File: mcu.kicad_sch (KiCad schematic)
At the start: 9 parts, among them SW1 SW_MEC_5E, U9 ESP32-S3-WROOM-1-N16R8

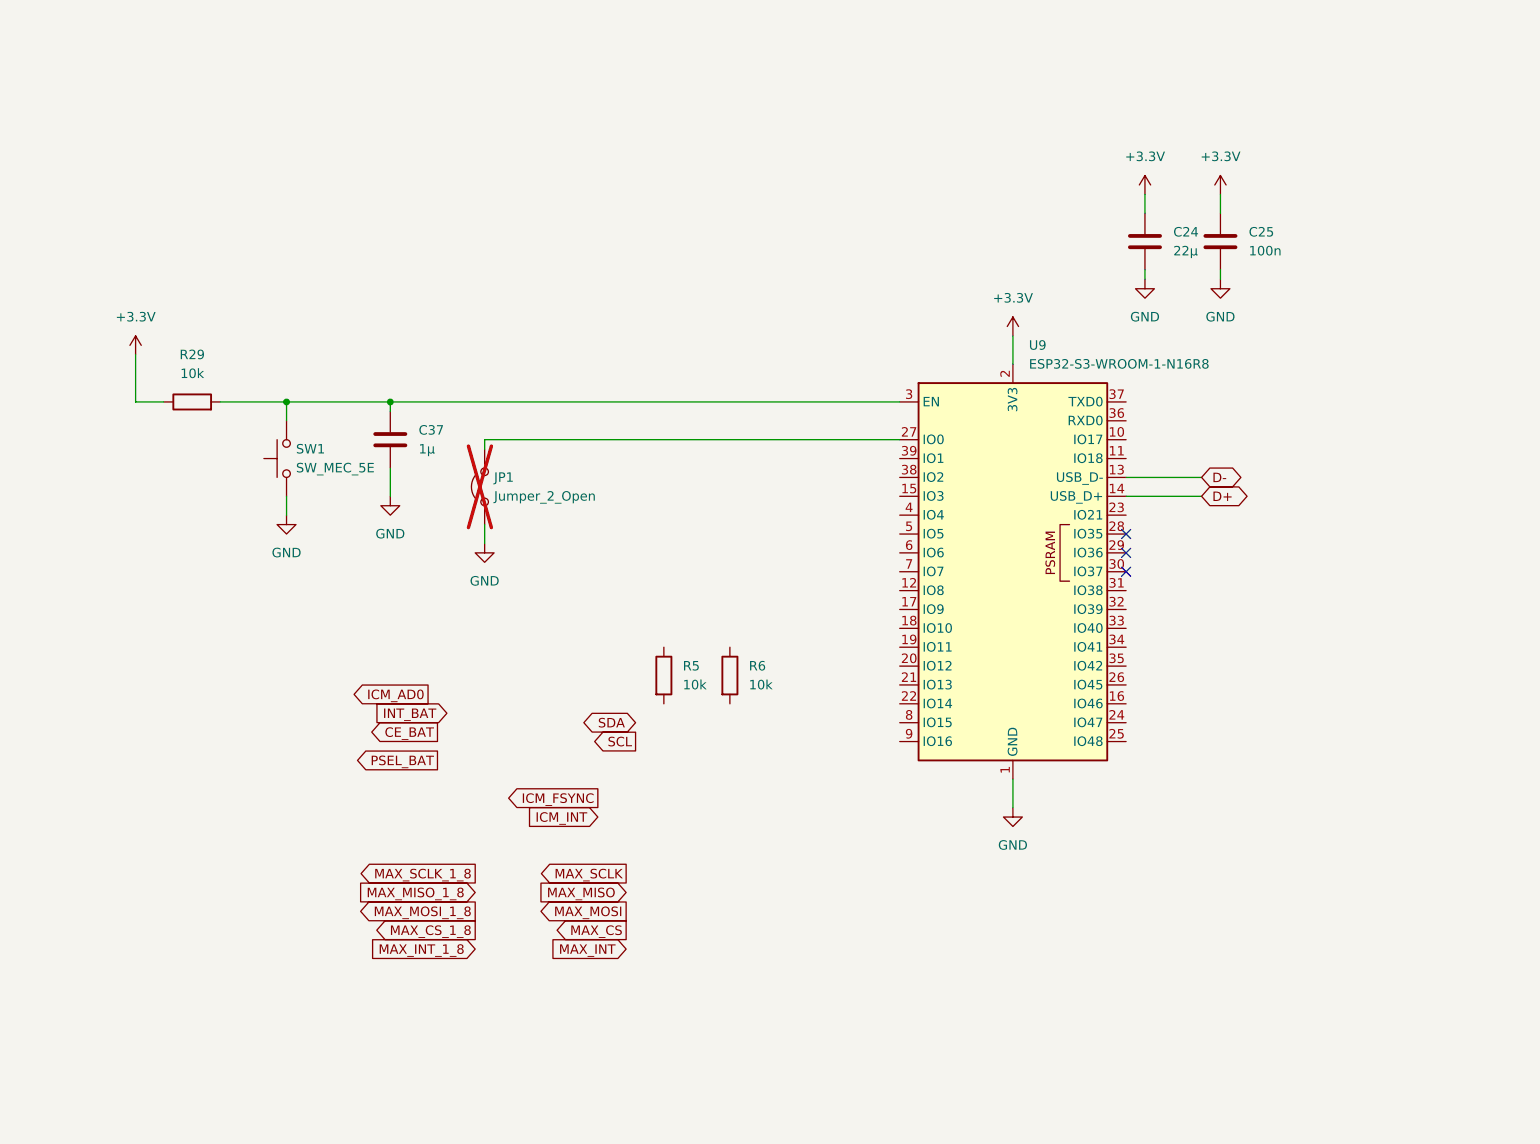
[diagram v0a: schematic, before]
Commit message: Routage complet
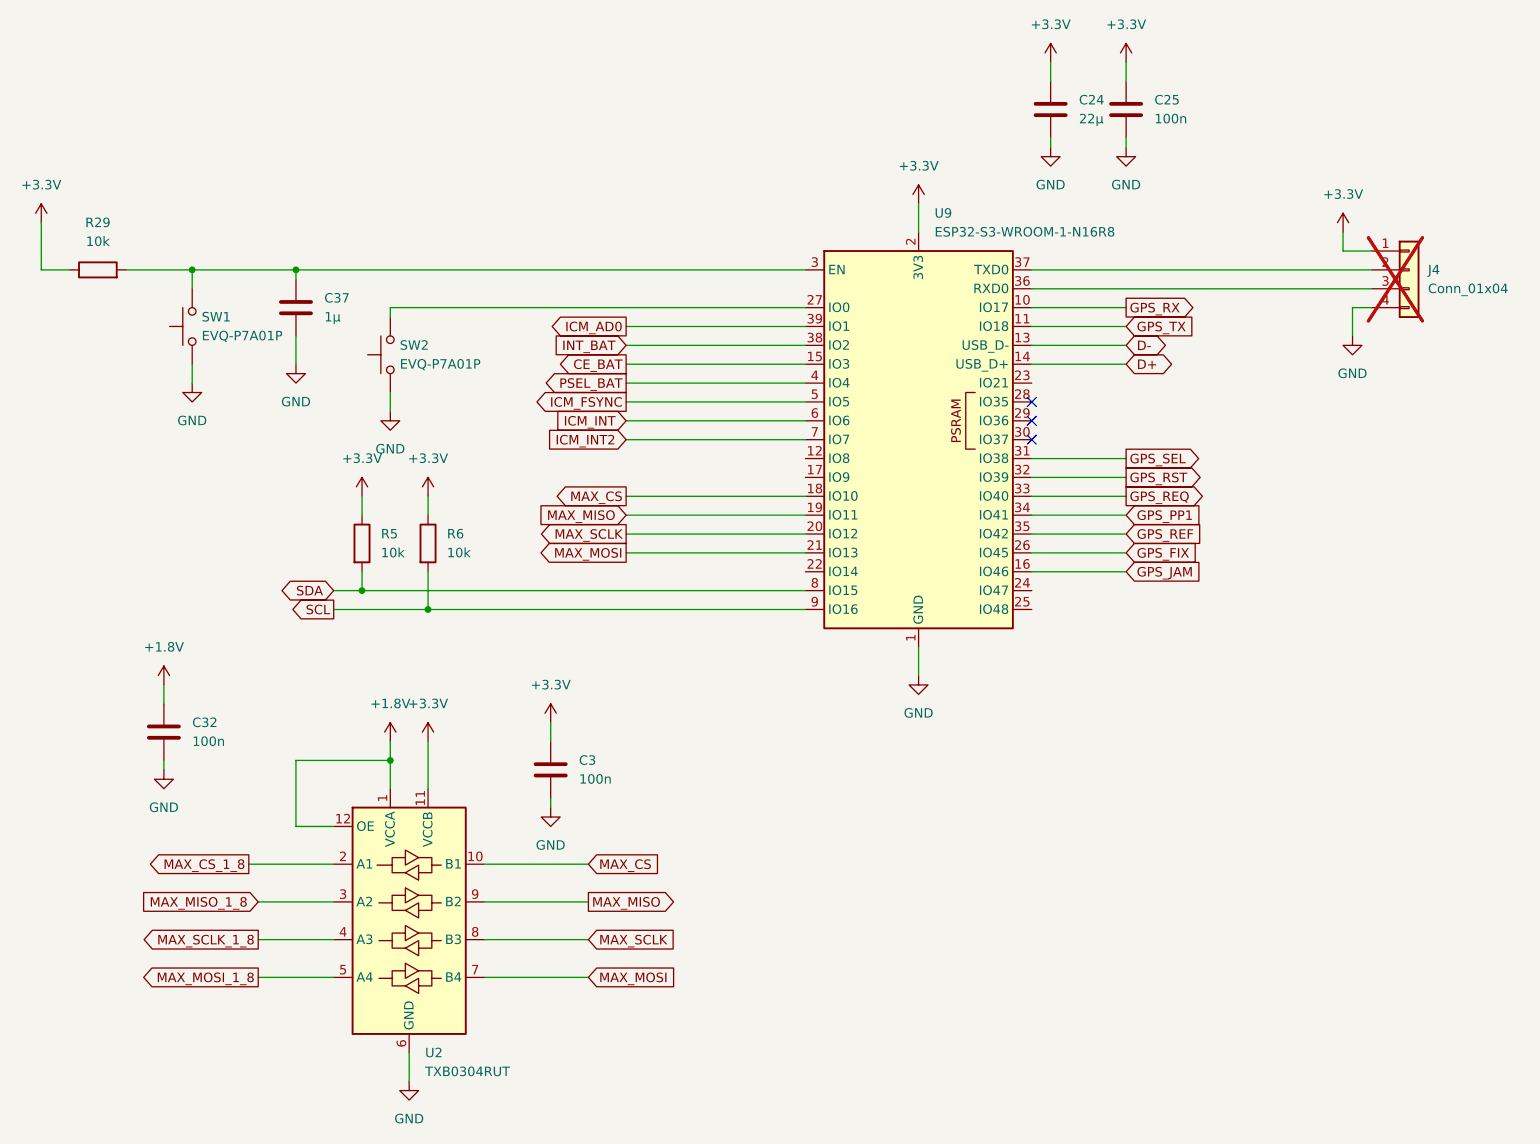
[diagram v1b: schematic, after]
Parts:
- removed JP1: Jumper_2_Open, Connector_PinHeader_2.54mm:PinHeader_1x02_P2.54mm_Vertical, symbol Jumper:Jumper_2_Open
- added C3, C32: 100n, Capacitor_SMD:C_0805_2012Metric, symbol Device:C
- added J4: Conn_01x04, Connector_PinHeader_1.27mm:PinHeader_1x04_P1.27mm_Vertical, symbol Connector_Generic:Conn_01x04
- added SW2: EVQ-P7A01P, Button_Switch_SMD:SW_SPST_EVQP7A, symbol Switch:SW_Omron_B3FS
- added U2: TXB0304RUT, Package_DFN_QFN:Texas_R-PUQFN-N12, symbol Logic_LevelTranslator:TXB0304RUT
- C24, C25: footprint (none) -> Capacitor_SMD:C_0805_2012Metric
- C37: footprint Capacitor_SMD:C_1206_3216Metric -> Capacitor_SMD:C_0805_2012Metric
- R29: footprint Resistor_SMD:R_1206_3216Metric -> Resistor_SMD:R_0805_2012Metric
- R5, R6: footprint (none) -> Resistor_SMD:R_0805_2012Metric
- SW1: value SW_MEC_5E -> EVQ-P7A01P; footprint Button_Switch_THT:SW_PUSH_6mm_H5mm -> Button_Switch_SMD:SW_SPST_EVQP7A
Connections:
- net +3.3V: now also R5.1, R6.1, C3.1, J4.1 (Pin_1), U2.11 (VCCB)
- net CE_BAT: now also U9.15 (IO3)
- net GND: now also C3.2, C32.2, J4.4 (Pin_4), SW2.1, U2.6 (GND)
- net ICM_AD0: now also U9.39 (IO1)
- net ICM_FSYNC: now also U9.5 (IO5)
- net ICM_INT: now also U9.6 (IO6)
- net INT_BAT: now also U9.38 (IO2)
- net MAX_CS: now also U9.18 (IO10), U2.10 (B1)
- net MAX_CS_1_8: now also U2.2 (A1)
- net MAX_MISO: now also U9.19 (IO11), U2.9 (B2)
- net MAX_MISO_1_8: now also U2.3 (A2)
- net MAX_MOSI: now also U9.21 (IO13), U2.7 (B4)
- net MAX_MOSI_1_8: now also U2.5 (A4)
- net MAX_SCLK: now also U9.20 (IO12), U2.8 (B3)
- net MAX_SCLK_1_8: now also U2.4 (A3)
- net PSEL_BAT: now also U9.4 (IO4)
- net SCL: now also R6.2, U9.9 (IO16)
- net SDA: now also R5.2, U9.8 (IO15)
- net GPS_RX: now reaches U9.10 (IO17)
- net GPS_TX: now reaches U9.11 (IO18)
- net GPS_JAM: now reaches U9.16 (IO46)
- net GPS_FIX: now reaches U9.26 (IO45)
- net at U9.27 (IO0): now also SW2.2
- net GPS_SEL: now reaches U9.31 (IO38)
- net GPS_RST: now reaches U9.32 (IO39)
- net GPS_REQ: now reaches U9.33 (IO40)
- net GPS_PP1: now reaches U9.34 (IO41)
- net GPS_REF: now reaches U9.35 (IO42)
- net at U9.36 (RXD0): now also J4.3 (Pin_3)
- net at U9.37 (TXD0): now also J4.2 (Pin_2)
- net ICM_INT2: now reaches U9.7 (IO7)
- new net +1.8V: C32.1, U2.1 (VCCA), U2.12 (OE)
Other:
- moved on the sheet: C24, C25, C37, R29, R5, R6, SW1, U9
